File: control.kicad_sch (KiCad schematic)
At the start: 0 parts

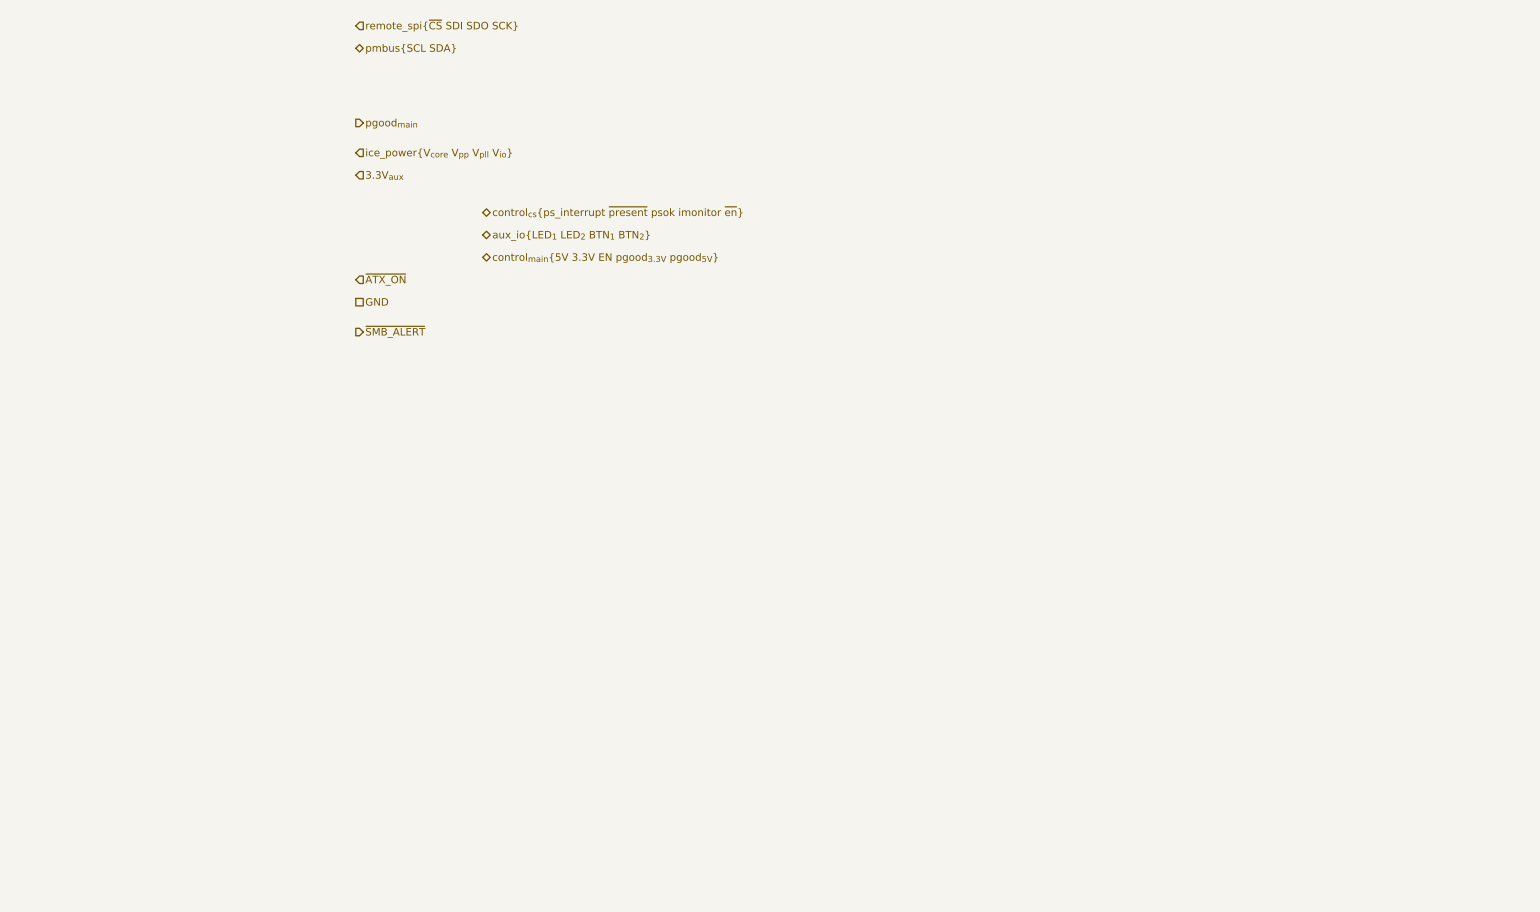
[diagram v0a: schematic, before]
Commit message: flesh out remote interface
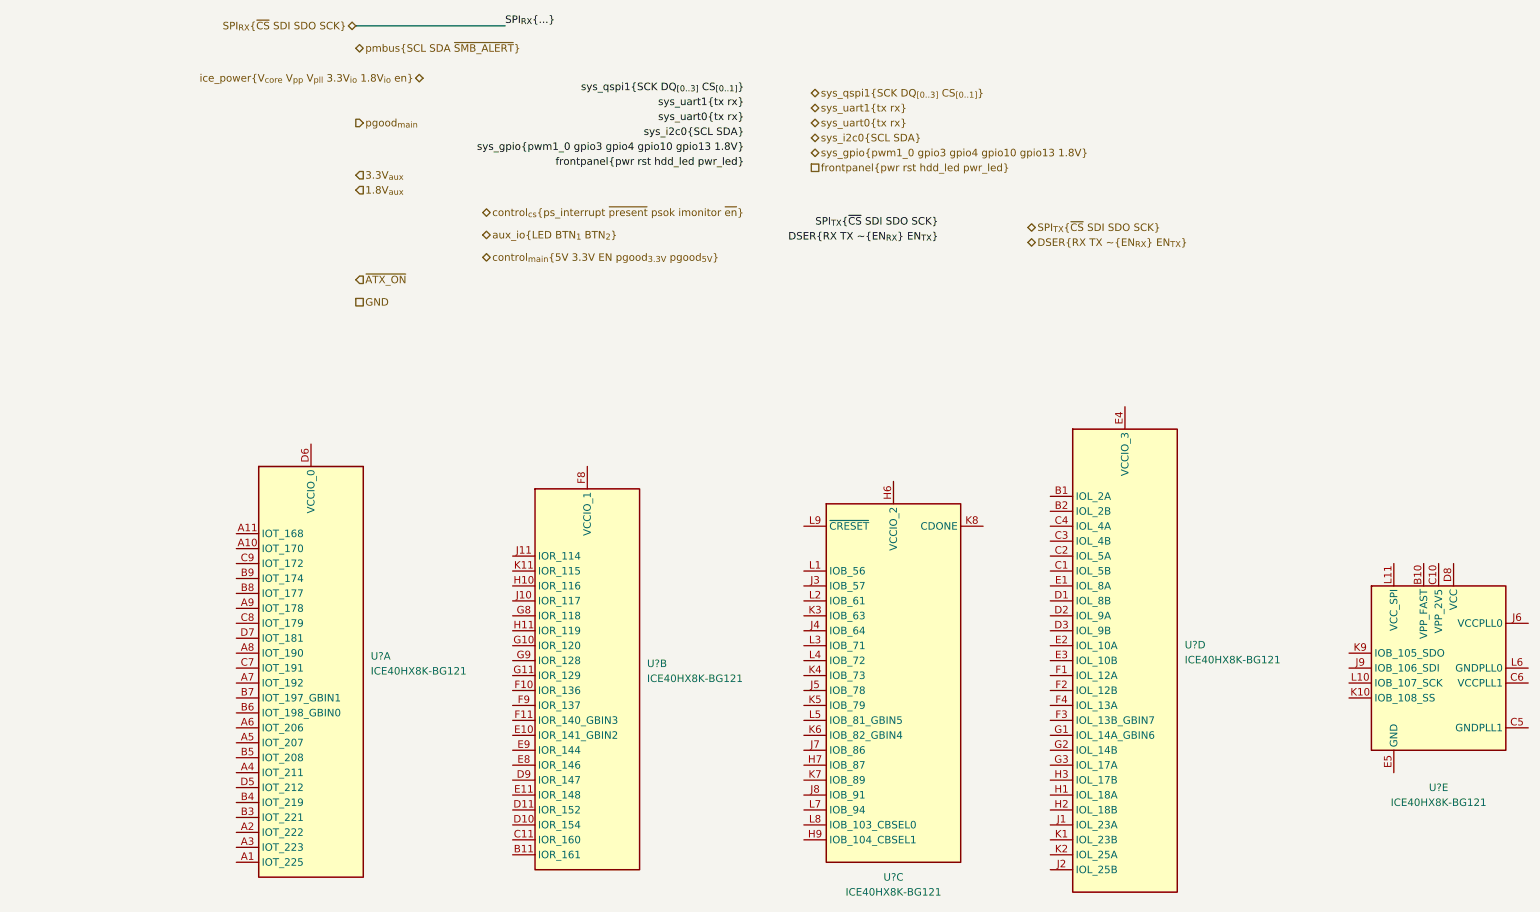
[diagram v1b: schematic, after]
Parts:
- added U? (x5): ICE40HX8K-BG121, Package_BGA:BGA-121_9.0x9.0mm_Layout11x11_P0.8mm_Ball0.4mm_Pad0.35mm_NSMD, symbol proj_sym:ICE40HX8K-BG121
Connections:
- new net: U?.D4 (VCC), U?.D8 (VCC), U?.H4 (VCC), U?.H8 (VCC)
- new net: U?.E5 (GND), U?.E6 (GND), U?.E7 (GND), U?.F5 (GND), U?.F6 (GND), U?.F7 (GND), U?.G5 (GND), U?.G6 (GND), U?.G7 (GND), U?.H5 (GND)
- new net: U?.E4 (VCCIO_3), U?.G4 (VCCIO_3)
